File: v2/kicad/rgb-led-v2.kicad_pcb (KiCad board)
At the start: 2 copper layers, 90 x 50 mm, 12 parts, among them SW1 SPST

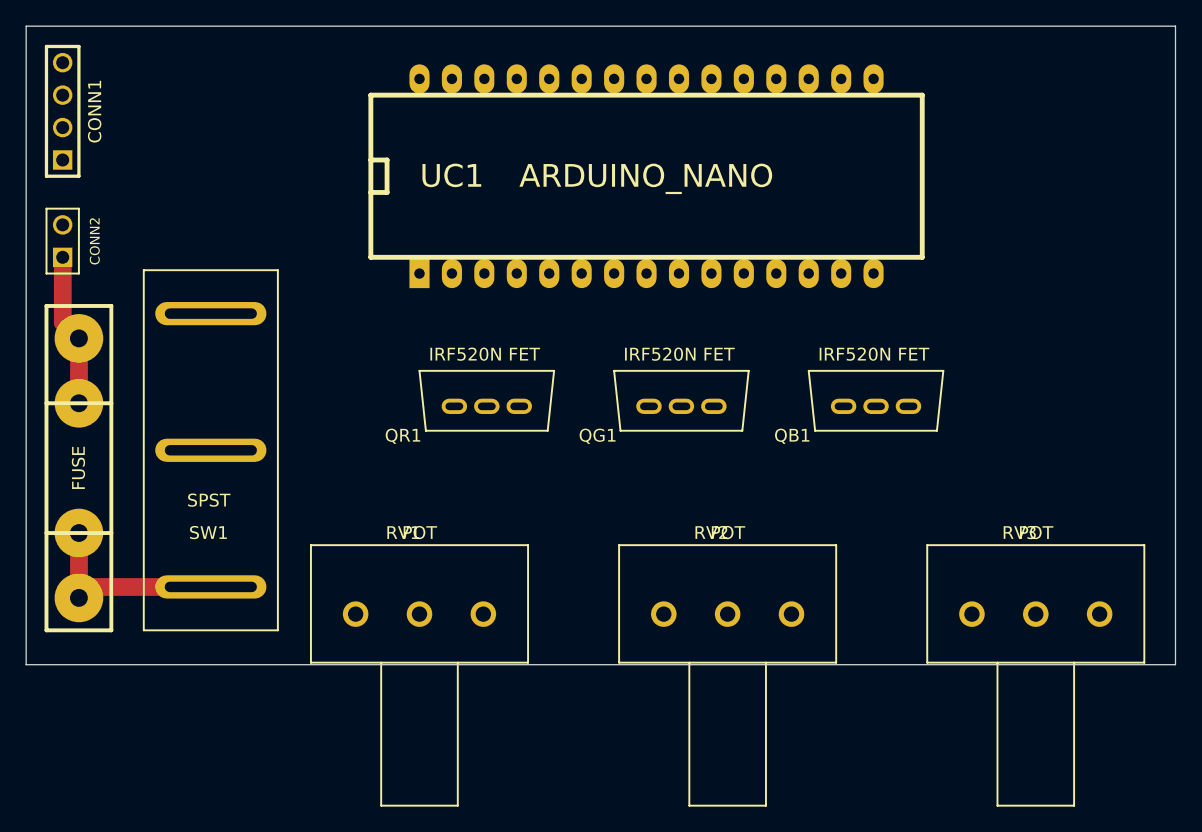
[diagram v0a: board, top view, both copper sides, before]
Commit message: [v2] PCB Routing
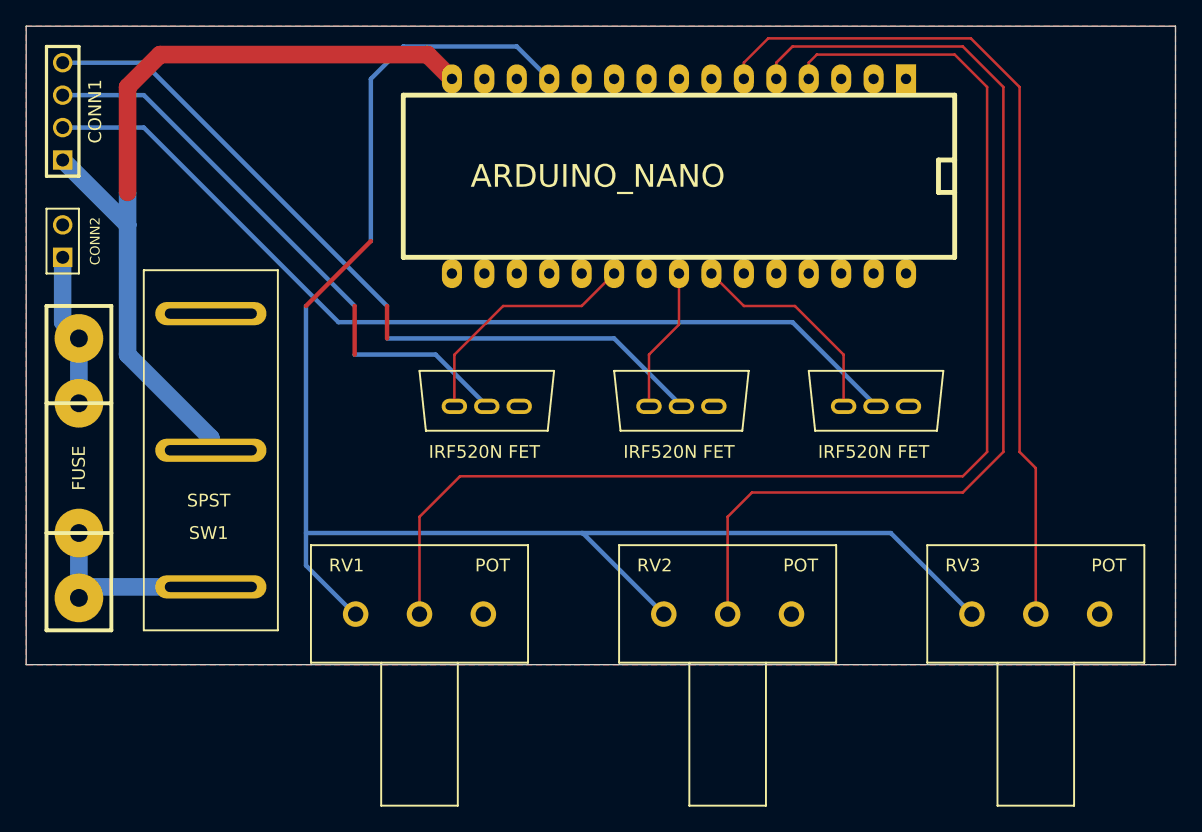
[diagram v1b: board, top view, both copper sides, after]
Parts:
- moved QB1 15.2 mm to (64.8, 47.0)
- moved QG1 15.2 mm to (80.0, 47.0)
- moved G*** 3.17 mm to (36.8, 28.6)
- turned UC1 to 180 degrees
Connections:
- CONN1 pad 1: N-000008 (its old number) -> N-000007
- SW1 pad 2: N-000008 (its old number) -> N-000007
- UC1 pad 15: (no net) -> N-000007
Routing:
- net N-000001: track 0.00 -> 125.6 mm, vias 0 -> 2
- net N-000003: track 0.00 -> 99.3 mm
- net N-000004: track 0.00 -> 80.8 mm
- net N-0000012: track 0.00 -> 72.8 mm
- net N-000005: track 0.00 -> 67.0 mm
- net N-000007: track 0.00 -> 65.6 mm, vias 0 -> 2
- net N-0000014: track 0.00 -> 61.1 mm, vias 0 -> 2
- net N-0000013: track 0.00 -> 45.6 mm, vias 0 -> 2
- net N-000009: track 0.00 -> 19.2 mm
- net N-0000011: track 0.00 -> 17.0 mm
- net N-0000010: track 0.00 -> 11.4 mm
- added copper zone on F.Cu, net GND
